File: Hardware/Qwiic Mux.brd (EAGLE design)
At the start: 40.6 x 54.6 mm, 78 parts, among them J1 SMD, J10 SMD, J11 PTH, J12 PTH, J13 PTH, J14 PTH, J2 SMD, J23 SMD, J24 SMD, J25 SMD, J26 SMD, J3 PTH, J4 PTH, J5 PTH, J6 PTH, J7 PTH, J8 SMD, J9 SMD, U2 PCA9548A, U3 3.3V/150mA, U4 2.8V/150mA

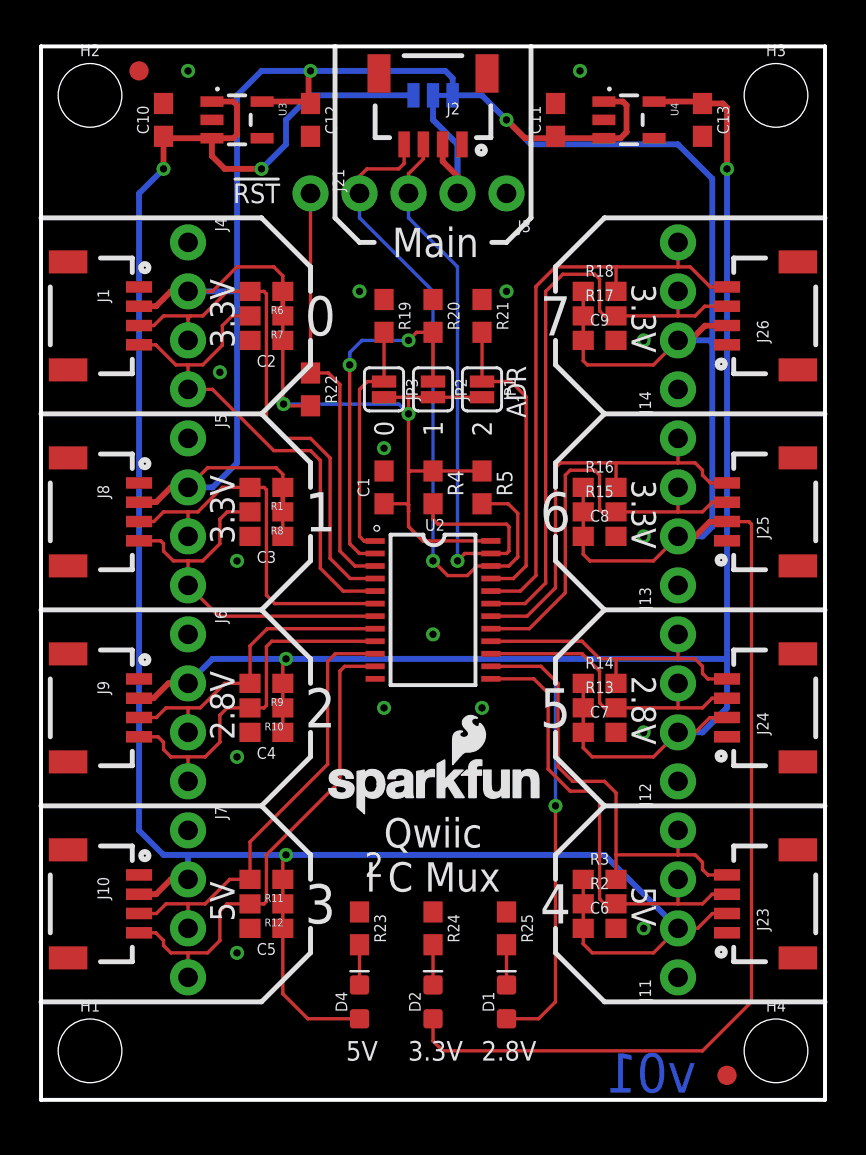
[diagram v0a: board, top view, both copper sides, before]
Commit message: Post design Review Changes
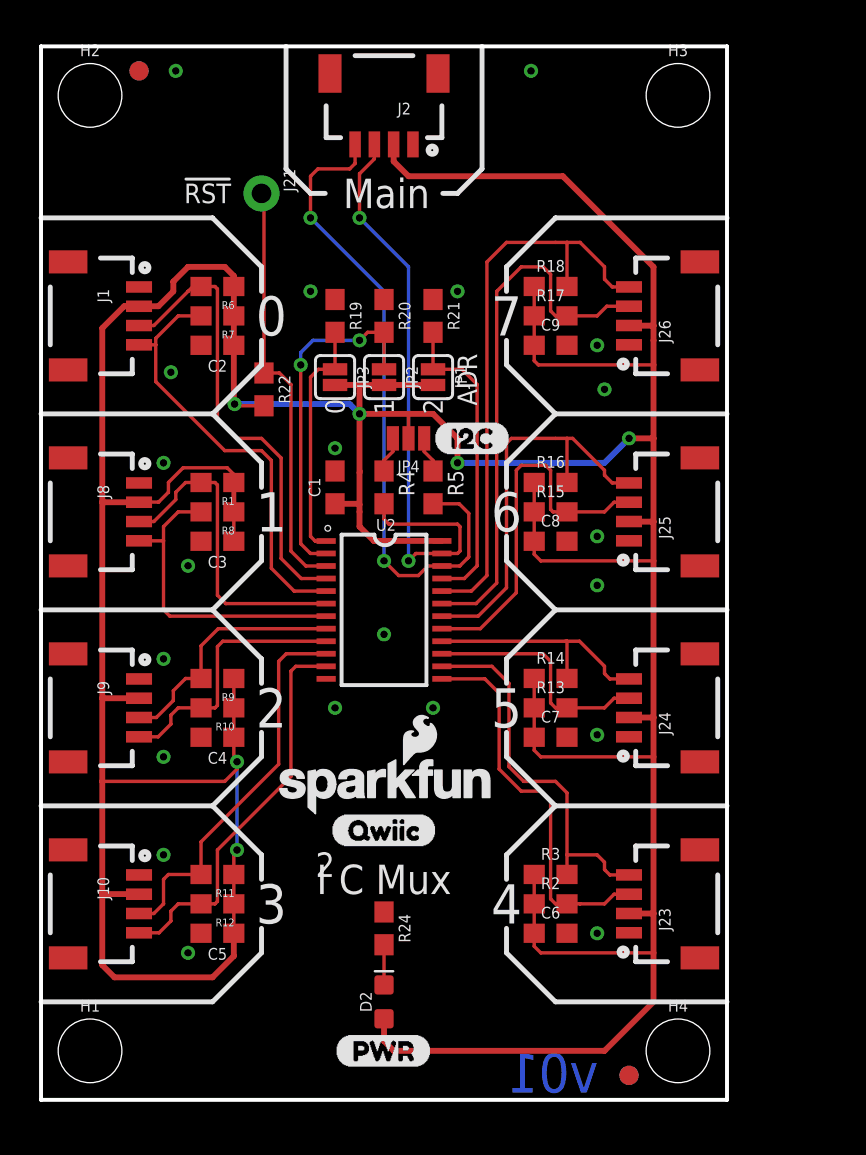
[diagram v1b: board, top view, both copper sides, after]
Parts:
- removed C10, C11, C13: 10uF, SparkFun-Capacitors:0603
- removed C12: 1.0uF, SparkFun-Capacitors:0603
- removed D1: GREEN, SparkFun-LED:LED-0603
- removed D4: BLUE, SparkFun-LED:LED-0603
- removed J11, J12, J13, J14, J3, J4, J5, J6, J7: PTH, SparkX:1X04_NO_SILK
- removed JP5: (no value), SparkFun-Jumpers:SMT-JUMPER_3_1-NC_TRACE_SILK
- removed R23, R25: 330, SparkFun-Resistors:0603
- removed U3: 3.3V/150mA, SparkFun-IC-Power:SOT23-5
- removed U4: 2.8V/150mA, SparkFun-IC-Power:SOT23-5
- added FD3, FD4: FIDUCIAL1X2, SparkFun-Aesthetics:FIDUCIAL-1X2
- added JP4: JUMPER-SMT_3_2-NC_PASTE_NO-SILK, SparkFun-Jumpers:SMT-JUMPER_3_2-NC_PASTE_NO-SILK
- added U$3: (no value), Labels-0_04:(PWR)
- added U$4: (no value), Labels-0_04:(QWIIC)
- added U$5: (no value), Labels-0_04:(I2C)
- D2: value Yellow -> RED
- R24: value 330 -> 1k
- U2: device SparkX:TSSOP28 -> SparkFun-IC-Logic:TSSOP28
- moved FD2 5.08 mm to (30.5, 1.27)
- moved H3 5.08 mm to (33.0, 52.1)
- moved H4 5.08 mm to (33.0, 2.54)
- moved J23 5.08 mm to (30.5, 10.2)
- moved J24 5.08 mm to (30.5, 20.3)
- moved J25 5.08 mm to (30.5, 30.5)
- moved J26 5.08 mm to (30.5, 40.6)
- moved JP1 2.62 mm to (20.3, 37.5)
- moved JP2 2.62 mm to (17.8, 37.5)
- moved JP3 2.62 mm to (15.2, 37.5)
- moved C2 2.55 mm to (9.14, 39.1)
- moved C3 2.55 mm to (9.14, 29.0)
- moved C4 2.55 mm to (9.14, 18.8)
- moved C5 2.55 mm to (9.14, 8.64)
- moved C6 2.55 mm to (26.4, 8.64)
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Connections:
- removed net 2.8V: C13.1, C4.1, C7.1, D1.A, J12.2, J24.2, J6.2, J9.2, R10.1, R13.1, R14.1, R9.1, U4.5
- removed net 5V: C10.1, C5.1, C6.1, D4.A, J10.2, J11.2, J23.2, J7.2, JP5.1, R11.1, R12.1, R2.1, R3.1, U3.1, U3.3
- removed net N$4: D4.C, R23.2
- removed net VIN: J2.2, J3.2, JP5.2
- new net N$2: JP4.3, R4.1
- net 3.3V: now also C4.1, C5.1, C6.1, C7.1, J10.2, J2.2, J23.2, J24.2, J9.2, JP4.2, R10.1, R11.1, R12.1, R13.1, R14.1, R2.1, R3.1, R9.1; no longer C11.1, C12.1, J13.2, J14.2, J4.2, J5.2, JP5.3, R4.1, R5.1, U3.5, U4.1, U4.3
- net GND: no longer C10.2, C11.2, C12.2, C13.2, J11.1, J12.1, J13.1, J14.1, J3.1, J4.1, J5.1, J6.1, J7.1, R23.1, R25.1, U3.2, U4.2
- net MAIN_SCL: no longer J3.4
- net MAIN_SDA: no longer J3.3
- net N$3: now also JP4.1, R5.1; no longer D1.C, R25.2
- net SCL0: no longer J4.4
- net SCL1: no longer J5.4
- net SCL2: no longer J6.4
- net SCL3: no longer J7.4
- net SCL4: no longer J11.4
- net SCL5: no longer J12.4
- net SCL6: no longer J13.4
- net SCL7: no longer J14.4
- net SDA0: no longer J4.3
- net SDA1: no longer J5.3
- net SDA2: no longer J6.3
- net SDA3: no longer J7.3
- net SDA4: no longer J11.3
- net SDA5: no longer J12.3
- net SDA6: no longer J13.3
- net SDA7: no longer J14.3
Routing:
- net 5V: track 115.1 -> 0.00 mm, vias 3 -> 0
- net 2.8V: track 105.9 -> 0.00 mm, vias 3 -> 0
- net 3.3V: track 213.8 -> 256.0 mm, vias 4 -> 6
- net VIN: track 8.46 -> 0.00 mm
- net SCL2: track 19.3 -> 13.8 mm
- net SCL3: track 25.9 -> 20.5 mm
- net SCL4: track 23.9 -> 19.8 mm
- net SCL0: track 26.4 -> 22.5 mm
- net SDA4: track 23.8 -> 20.0 mm
- net SDA2: track 16.6 -> 12.9 mm
- net SDA5: track 15.8 -> 12.3 mm
- net SCL1: track 19.8 -> 16.4 mm
- net SDA0: track 27.6 -> 24.3 mm
- net SDA7: track 31.5 -> 28.2 mm
- net SDA6: track 22.6 -> 19.3 mm
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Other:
- board size 40.6 x 54.6 mm -> 35.6 x 54.6 mm
- board text added: "I C Mux"
- board text added: "Measures in Inches"
- board text removed: "2.8V"
- board text removed: "3.3V"
- board text removed: "5V"
- board text removed: "GND"
- board text removed: "Qwiic I C Mux"
- board text removed: "SCL"
- board text removed: "SCL0"
- board text removed: "SCL1"
- board text removed: "SCL2"
- board text removed: "SCL3"
- board text removed: "SCL4"
- board text removed: "SCL5"
- board text removed: "SCL6"
- board text removed: "SCL7"
- board text removed: "SDA"
- board text removed: "SDA0"
- board text removed: "SDA1"
- board text removed: "SDA2"
- board text removed: "SDA3"
- board text removed: "SDA4"
- board text removed: "SDA5"
- board text removed: "SDA6"
- board text removed: "SDA7"
- board text removed: "VIN"
- board text removed: "VIN SEL"
